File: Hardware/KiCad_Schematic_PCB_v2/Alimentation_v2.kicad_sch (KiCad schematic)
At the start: 12 parts, among them J501 JST_switch, SW501 SW_SPDT, U501 AZ1117-5.0, U502 MCP1802x-xx02xOT

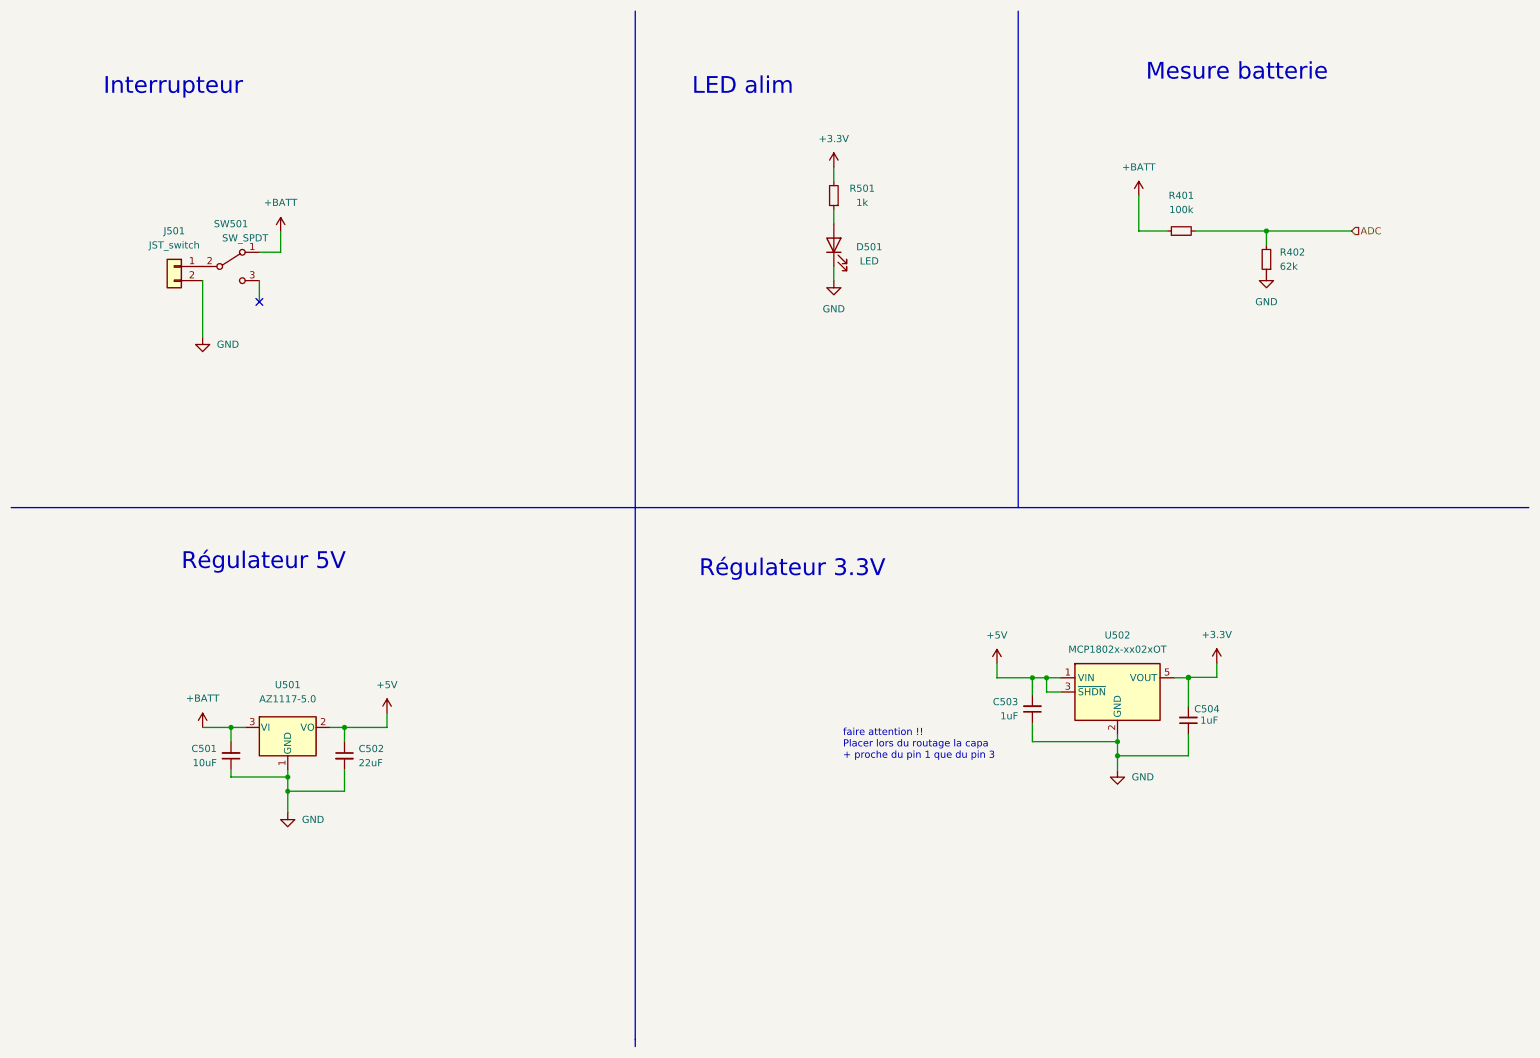
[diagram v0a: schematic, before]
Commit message: Final placement
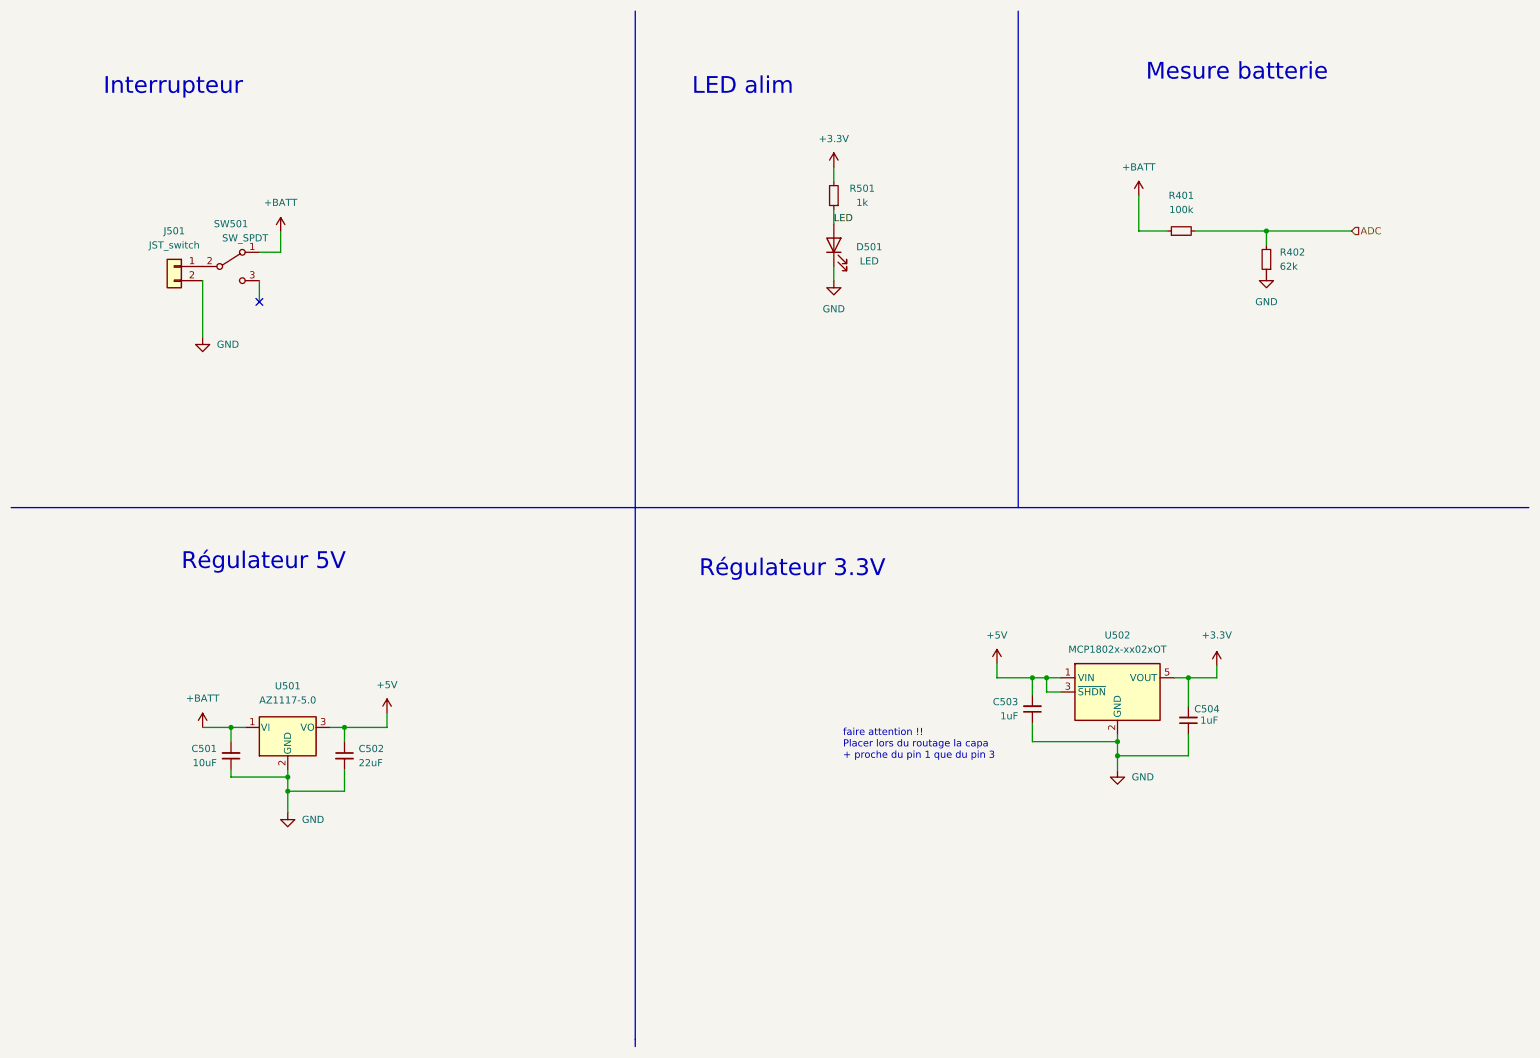
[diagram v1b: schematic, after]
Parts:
- removed U501: AZ1117-5.0, Package_TO_SOT_SMD:SOT-223-3_TabPin2, symbol Regulator_Linear:AZ1117-5.0
- added U501: AZ1117-5.0, Package_TO_SOT_SMD:SOT-223-3_TabPin2, symbol Regulator_Linear:LT1129-3.3_SOT223
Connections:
- net +3.3V: now also C504.2, U502.5 (VOUT)
- net +5V: now also U501.3 (VO)
- net +BATT: now also U501.1 (VI)
- net GND: now also U501.2 (GND)
- net LED: now reaches D501.2 (A), R501.1
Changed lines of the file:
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@@
   (junction (at 72.39 140.97) (diameter 0) (color 0 0 0 0)
-  )
-  (junction (at 223.5209 131.9982) (diameter 0) (color 0 0 0 0)
   )
   (junction (at 198.12 132.08) (diameter 0) (color 0 0 0 0)
@@
     (stroke (width 0) (type default) (color 0 0 0 0))
   )
+  (wire (pts (xy 228.6 132.08) (xy 228.6 129.9464))
+    (stroke (width 0) (type default) (color 0 0 0 0))
+  )
   (wire (pts (xy 52.07 148.59) (xy 52.07 149.86))
     (stroke (width 0) (type default) (color 0 0 0 0))
@@
     (stroke (width 0) (type default) (color 0 0 0 0))
   )
-  (wire (pts (xy 228.6009 129.4582) (xy 228.6009 131.9982))
-    (stroke (width 0) (type default) (color 0 0 0 0))
-  )
   (wire (pts (xy 72.39 148.59) (xy 72.39 152.4))
     (stroke (width 0) (type default) (color 0 0 0 0))
@@
     (stroke (width 0) (type default) (color 0 0 0 0))
   )
+  (wire (pts (xy 72.39 140.97) (xy 72.39 143.51))
+    (stroke (width 0) (type default) (color 0 0 0 0))
+  )
+  (wire (pts (xy 223.52 132.08) (xy 228.6 132.08))
+    (stroke (width 0) (type default) (color 0 0 0 0))
+  )
+  (wire (pts (xy 237.49 52.07) (xy 252.73 52.07))
+    (stroke (width 0) (type default) (color 0 0 0 0))
+  )
+  (wire (pts (xy 210.82 146.05) (xy 210.82 143.51))
+    (stroke (width 0) (type default) (color 0 0 0 0))
+  )
+  (wire (pts (xy 223.52 132.08) (xy 223.52 137.16))
+    (stroke (width 0) (type default) (color 0 0 0 0))
+  )
+  (wire (pts (xy 219.71 52.07) (xy 214.63 52.07))
+    (stroke (width 0) (type default) (color 0 0 0 0))
+  )
+  (wire (pts (xy 46.99 140.97) (xy 52.07 140.97))
+    (stroke (width 0) (type default) (color 0 0 0 0))
+  )
+  (wire (pts (xy 160.02 58.42) (xy 160.02 60.96))
+    (stroke (width 0) (type default) (color 0 0 0 0))
+  )
+  (wire (pts (xy 72.39 140.97) (xy 80.01 140.97))
+    (stroke (width 0) (type default) (color 0 0 0 0))
+  )
+  (wire (pts (xy 52.07 149.86) (xy 62.23 149.86))
+    (stroke (width 0) (type default) (color 0 0 0 0))
+  )
+  (wire (pts (xy 223.52 142.24) (xy 223.52 146.05))
+    (stroke (width 0) (type default) (color 0 0 0 0))
+  )
+  (polyline (pts (xy 193.04 12.7) (xy 193.04 101.6))
+    (stroke (width 0) (type default) (color 0 0 0 0))
+  )
+  (wire (pts (xy 62.23 156.21) (xy 62.23 152.4))
+    (stroke (width 0) (type default) (color 0 0 0 0))
+  )
+  (wire (pts (xy 224.79 52.07) (xy 237.49 52.07))
+    (stroke (width 0) (type default) (color 0 0 0 0))
+  )
+  (wire (pts (xy 72.39 152.4) (xy 62.23 152.4))
+    (stroke (width 0) (type default) (color 0 0 0 0))
+  )
+  (polyline (pts (xy 12.7 101.6) (xy 284.48 101.6))
+    (stroke (width 0) (type default) (color 0 0 0 0))
+  )
+  (wire (pts (xy 160.02 48.26) (xy 160.02 50.8))
+    (stroke (width 0) (type default) (color 0 0 0 0))
+  )
+  (wire (pts (xy 223.52 146.05) (xy 210.82 146.05))
+    (stroke (width 0) (type default) (color 0 0 0 0))
+  )
   (wire (pts (xy 220.98 132.08) (xy 223.52 132.08))
-    (stroke (width 0) (type default) (color 0 0 0 0))
-  )
-  (wire (pts (xy 72.39 140.97) (xy 72.39 143.51))
-    (stroke (width 0) (type default) (color 0 0 0 0))
-  )
-  (wire (pts (xy 237.49 52.07) (xy 252.73 52.07))
-    (stroke (width 0) (type default) (color 0 0 0 0))
-  )
-  (wire (pts (xy 210.82 146.05) (xy 210.82 143.51))
-    (stroke (width 0) (type default) (color 0 0 0 0))
-  )
-  (wire (pts (xy 223.52 132.08) (xy 223.52 137.16))
-    (stroke (width 0) (type default) (color 0 0 0 0))
-  )
-  (wire (pts (xy 219.71 52.07) (xy 214.63 52.07))
-    (stroke (width 0) (type default) (color 0 0 0 0))
-  )
-  (wire (pts (xy 46.99 140.97) (xy 52.07 140.97))
-    (stroke (width 0) (type default) (color 0 0 0 0))
-  )
-  (wire (pts (xy 160.02 58.42) (xy 160.02 60.96))
-    (stroke (width 0) (type default) (color 0 0 0 0))
-  )
-  (wire (pts (xy 72.39 140.97) (xy 80.01 140.97))
-    (stroke (width 0) (type default) (color 0 0 0 0))
-  )
-  (wire (pts (xy 52.07 149.86) (xy 62.23 149.86))
-    (stroke (width 0) (type default) (color 0 0 0 0))
-  )
-  (wire (pts (xy 223.52 142.24) (xy 223.52 146.05))
-    (stroke (width 0) (type default) (color 0 0 0 0))
-  )
-  (polyline (pts (xy 193.04 12.7) (xy 193.04 101.6))
-    (stroke (width 0) (type default) (color 0 0 0 0))
-  )
-  (wire (pts (xy 62.23 156.21) (xy 62.23 152.4))
-    (stroke (width 0) (type default) (color 0 0 0 0))
-  )
-  (wire (pts (xy 224.79 52.07) (xy 237.49 52.07))
-    (stroke (width 0) (type default) (color 0 0 0 0))
-  )
-  (wire (pts (xy 72.39 152.4) (xy 62.23 152.4))
-    (stroke (width 0) (type default) (color 0 0 0 0))
-  )
-  (polyline (pts (xy 12.7 101.6) (xy 284.48 101.6))
-    (stroke (width 0) (type default) (color 0 0 0 0))
-  )
-  (wire (pts (xy 160.02 48.26) (xy 160.02 50.8))
-    (stroke (width 0) (type default) (color 0 0 0 0))
-  )
-  (wire (pts (xy 223.52 146.05) (xy 210.82 146.05))
-    (stroke (width 0) (type default) (color 0 0 0 0))
-  )
-  (wire (pts (xy 223.5209 131.9982) (xy 228.6009 131.9982))
     (stroke (width 0) (type default) (color 0 0 0 0))
   )
@@
     (effects (font (size 3 3)) (justify left bottom))
   )
+  (label "LED" (at 160.02 50.8 0)
+    (effects (font (size 1.27 1.27)) (justify left bottom))
+  )
   (hierarchical_label "ADC" (shape input) (at 252.73 52.07 0)
     (effects (font (size 1.27 1.27)) (justify left))
@@
     (pin "2")
   )
-  (symbol (lib_id "Regulator_Linear:AZ1117-5.0") (at 62.23 140.97 0) (unit 1)
-    (in_bom yes) (on_board yes) (fields_autoplaced)
-    (property "Reference" "U501" (id 0) (at 62.23 133.35 0))
-    (property "Value" "AZ1117-5.0" (id 1) (at 62.23 135.89 0))
-    (property "Footprint" "Package_TO_SOT_SMD:SOT-223-3_TabPin2" (id 2) (at 62.23 134.62 0)
-      (effects (font (size 1.27 1.27) italic) hide)
-    )
-    (property "Datasheet" "https://www.diodes.com/assets/Datasheets/AZ1117.pdf" (id 3) (at 62.23 140.97 0)
-      (effects (font (size 1.27 1.27)) hide)
-    )
-    (pin "1")
-    (pin "2")
-    (pin "3")
-  )
   (symbol (lib_id "power:+BATT") (at 214.63 45.72 0) (unit 1)
     (in_bom yes) (on_board yes) (fields_autoplaced)
@@
     )
     (pin "1")
+  )
+  (symbol (lib_id "Regulator_Linear:LT1129-3.3_SOT223") (at 62.23 140.97 0) (unit 1)
+    (in_bom yes) (on_board yes) (fields_autoplaced)
+    (property "Reference" "U501" (id 0) (at 62.23 133.5532 0))
+    (property "Value" "AZ1117-5.0" (id 1) (at 62.23 136.0932 0))
+    (property "Footprint" "Package_TO_SOT_SMD:SOT-223-3_TabPin2" (id 2) (at 62.23 135.255 0)
+      (effects (font (size 1.27 1.27) italic) hide)
+    )
+    (property "Datasheet" "https://www.analog.com/media/en/technical-documentation/data-sheets/112935ff.pdf" (id 3) (at 62.23 142.24 0)
+      (effects (font (size 1.27 1.27)) hide)
+    )
+    (pin "1")
+    (pin "2")
+    (pin "3")
   )
   (symbol (lib_id "Connector_Generic:Conn_01x02") (at 41.91 58.42 0) (mirror y) (unit 1)
@@
     (pin "1")
   )
-  (symbol (lib_id "power:+3.3V") (at 228.6009 129.4582 0) (unit 1)
-    (in_bom yes) (on_board yes) (fields_autoplaced)
-    (property "Reference" "#PWR0410" (id 0) (at 228.6009 133.2682 0)
-      (effects (font (size 1.27 1.27)) hide)
-    )
-    (property "Value" "+3.3V" (id 1) (at 228.6009 124.3782 0))
-    (property "Footprint" "" (id 2) (at 228.6009 129.4582 0)
-      (effects (font (size 1.27 1.27)) hide)
-    )
-    (property "Datasheet" "" (id 3) (at 228.6009 129.4582 0)
-      (effects (font (size 1.27 1.27)) hide)
-    )
-    (pin "1")
-  )
   (symbol (lib_id "Device:C_Small") (at 72.39 146.05 0) (unit 1)
     (in_bom yes) (on_board yes) (fields_autoplaced)
@@
       (effects (font (size 1.27 1.27)) hide)
     )
+    (pin "1")
+  )
+  (symbol (lib_id "power:+3.3V") (at 228.6 129.9464 0) (unit 1)
+    (in_bom yes) (on_board yes) (fields_autoplaced)
+    (property "Reference" "#PWR0102" (id 0) (at 228.6 133.7564 0)
+      (effects (font (size 1.27 1.27)) hide)
+    )
+    (property "Value" "+3.3V" (id 1) (at 228.6 124.46 0))
+    (property "Footprint" "" (id 2) (at 228.6 129.9464 0)
+      (effects (font (size 1.27 1.27)) hide)
+    )
+    (property "Datasheet" "" (id 3) (at 228.6 129.9464 0)
+      (effects (font (size 1.27 1.27)) hide)
+    )
